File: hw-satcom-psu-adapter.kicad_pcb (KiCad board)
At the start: 2 copper layers, 89.2 x 45 mm, 37 parts, among them J1 Conn_01x04, J2 XT30, J3 XT30, J4 Conn_01x06_MountingPin, J5 s, U1 Brick-DCDC

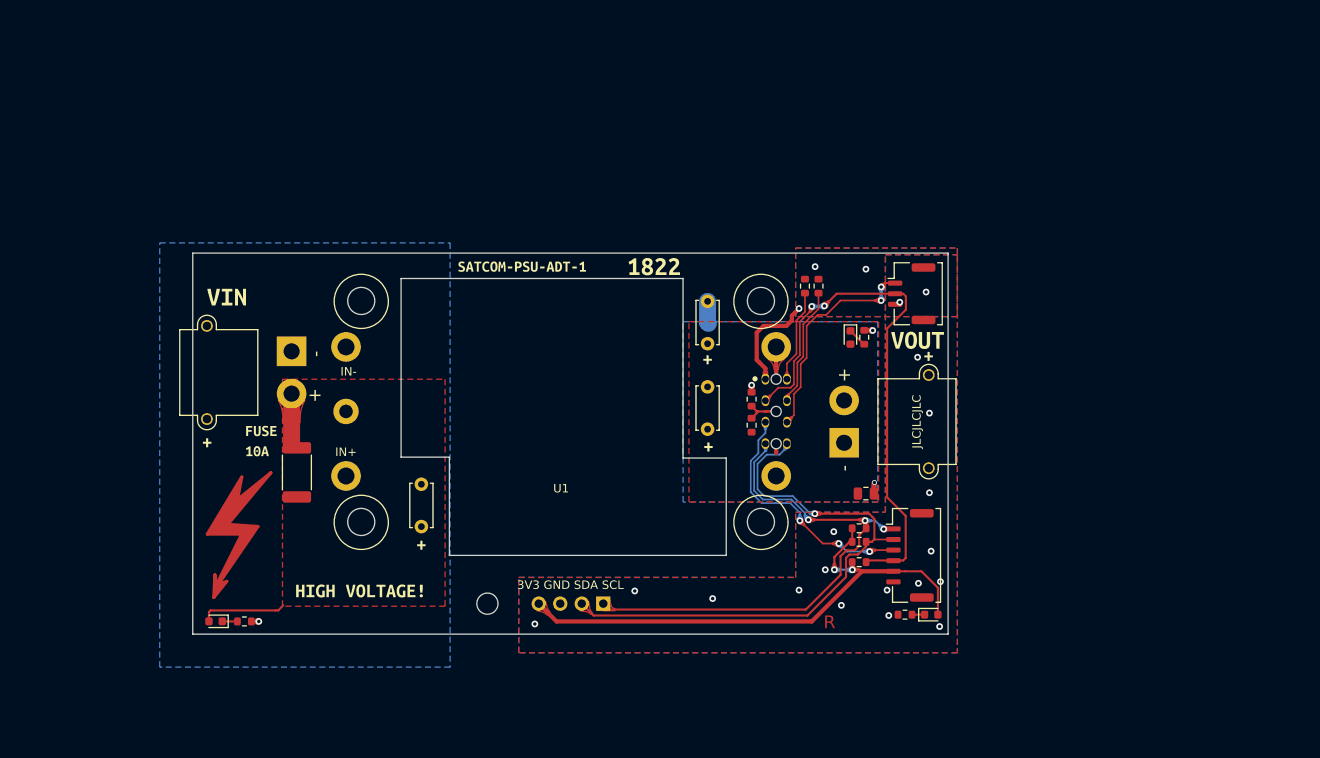
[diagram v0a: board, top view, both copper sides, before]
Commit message: ATX
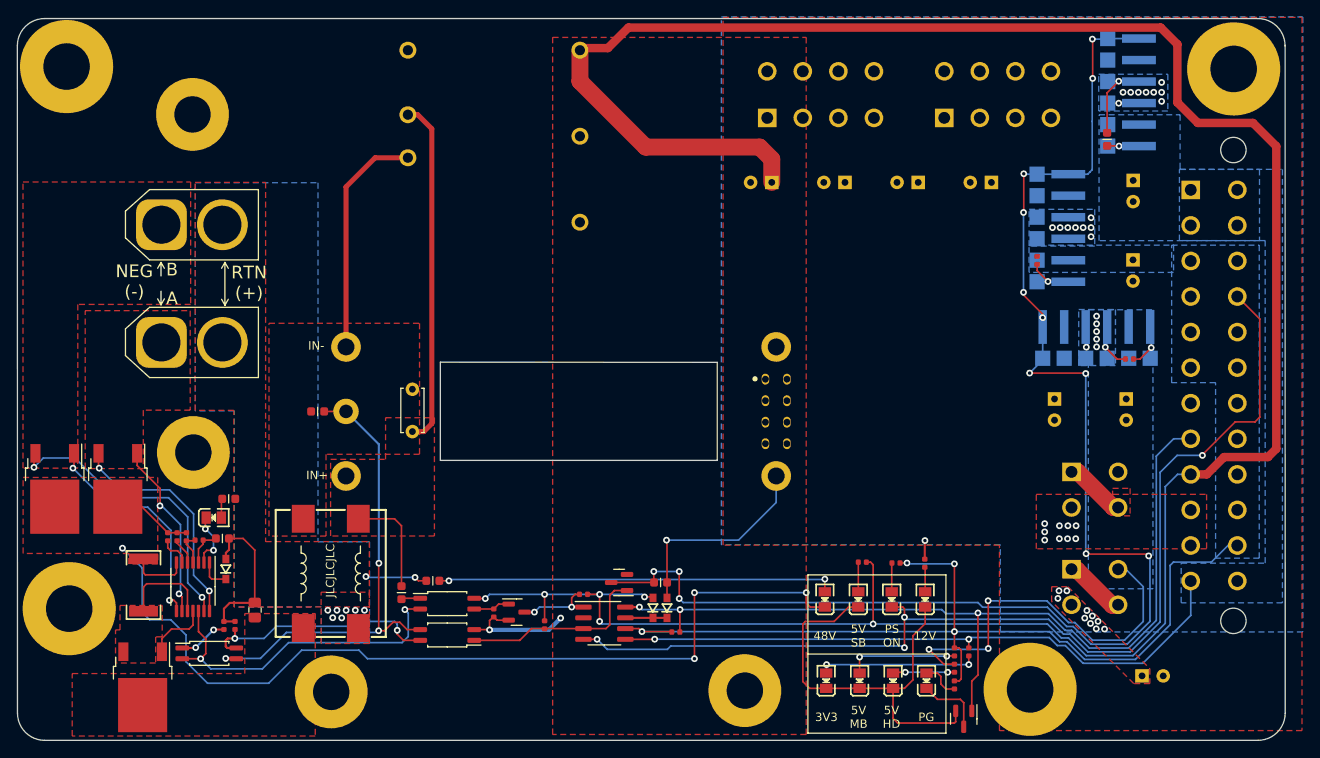
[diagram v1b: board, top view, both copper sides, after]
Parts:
- removed C2, C3: 470uF/50V, Capacitor_THT:C_Disc_D5.0mm_W2.5mm_P5.00mm
- removed C4: 1uF/50V, Capacitor_SMD:C_0805_2012Metric
- removed F1: 10A, Fuse:Fuse_2512_6332Metric
- removed H1: MountingHole, MountingHole:MountingHole_2.5mm
- removed R10, R9: NC, Resistor_SMD:R_0603_1608Metric
- removed REF**: Symbol_HighVoltage_Type1_CopperTop_Big, Symbol:Symbol_HighVoltage_Type1_CopperTop_Big
- removed kibuzzard-6276051F: G***, kibuzzard-6276051F
- removed kibuzzard-6276052C: G***, kibuzzard-6276052C
- removed kibuzzard-62760583 (x5): G***, kibuzzard-62760583
- removed kibuzzard-62760647: G***, kibuzzard-62760647
- removed kibuzzard-62760724: G***, kibuzzard-62760724
- removed kibuzzard-62760775: G***, kibuzzard-62760775
- added C10: 470uF/25V, Capacitor_THT:CP_Radial_D6.3mm_P2.50mm, B.Cu at (183.4, 69.8)
- added C12: 470uF/25V, Capacitor_THT:CP_Radial_D6.3mm_P2.50mm, B.Cu at (208.2, 95.4)
- added C13: 470uF/25V, Capacitor_THT:CP_Radial_D6.3mm_P2.50mm, B.Cu at (218.5, 128.1)
- added C14: 100nF/100V, lc:0805_C, F.Cu at (113.7, 120.4)
- added C15: 470uF/25V, Capacitor_THT:CP_Radial_D6.3mm_P2.50mm, B.Cu at (217.5, 69.6)
- added C16: 470uF/25V, Capacitor_THT:CP_Radial_D6.3mm_P2.50mm, B.Cu at (217.4, 79.0)
- added C17: 470uF/25V, Capacitor_THT:CP_Radial_D6.3mm_P2.50mm, B.Cu at (216.6, 95.4)
- added C5: 47nF, lc:0402_C, F.Cu at (104.5, 111.7)
- added C6: 10nF, lc:0402_C, F.Cu at (103.5, 111.7)
- added C7: 470uF/25V, Capacitor_THT:CP_Radial_D6.3mm_P2.50mm, B.Cu at (200.7, 69.8)
- added C8: 470uF/25V, Capacitor_THT:CP_Radial_D6.3mm_P2.50mm, B.Cu at (192.1, 69.8)
- added C9: 470uF/25V, Capacitor_THT:CP_Radial_D6.3mm_P2.50mm, B.Cu at (174.8, 69.8)
- added D10: Green, lc:0805_LED_S1_NUM, F.Cu at (189.1, 128.7)
- added D11: Blue, lc:0805_LED_S1_NUM, F.Cu at (193.1, 128.7)
- added D12: Blue, lc:0805_LED_S1_NUM, F.Cu at (188.9, 119.1)
- added D4: Yellow, lc:0805_LED_S1_NUM, F.Cu at (181.1, 119.1)
- added D5: Yellow, lc:0805_LED_S1_NUM, F.Cu at (185.0, 119.1)
- added D6: 1N5819WS, lc:SOD-323, F.Cu at (162.4, 120.1)
- added D7: 1N5819WS, lc:SOD-323, F.Cu at (160.8, 120.1)
- added D8: Green, lc:0805_LED_S1_NUM, F.Cu at (181.2, 128.7)
- added D9: Green, lc:0805_LED_S1_NUM, F.Cu at (185.2, 128.7)
- added FL1: ACM1513F-551T100, t123yh:ACM1513, F.Cu at (122.7, 116.0)
- added G***: LOGO, LOGO, F.Cu at (160.6, 93.1)
- added H2: SMTSO-M3, MountingHole:MountingHole_4.3mm_M4_Pad, B.Cu at (106.5, 101.8)
- added H3: SMTSO-M3, MountingHole:MountingHole_4.3mm_M4_Pad, B.Cu at (106.4, 61.8)
- added H4: SMTSO-632, MountingHole:MountingHole_5.5mm_Pad, B.Cu at (229.3, 56.5)
- added H5: SMTSO-632, MountingHole:MountingHole_5.5mm_Pad, B.Cu at (91.8, 120.2)
- added H6: SMTSO-632, MountingHole:MountingHole_5.5mm_Pad, B.Cu at (91.5, 56.2)
- added H7: SMTSO-632, MountingHole:MountingHole_5.5mm_Pad, B.Cu at (205.3, 129.7)
- added H8: SMTSO-M3, MountingHole:MountingHole_4.3mm_M4_Pad, F.Cu at (171.6, 129.9)
- added H9: SMTSO-M3, MountingHole:MountingHole_4.3mm_M4_Pad, F.Cu at (122.8, 130.0)
- added J_CPU1: Conn_02x04_Top_Bottom, t123yh:ATX-8P, B.Cu at (201.4, 59.5)
- added J_CPU2: Conn_02x04_Top_Bottom, t123yh:ATX-8P, B.Cu at (180.5, 59.5)
- added Q1: NCE0140K2, Package_TO_SOT_SMD:TO-252-2, F.Cu at (90.1, 106.0)
- added Q2: NCE0140K2, Package_TO_SOT_SMD:TO-252-2, F.Cu at (100.5, 129.5)
- added Q3: NCE0140K2, Package_TO_SOT_SMD:TO-252-2, F.Cu at (97.5, 106.0)
- added Q4: 2N7002, Package_TO_SOT_SMD:SOT-23, F.Cu at (144.7, 120.6)
- added Q5: 2N7002, Package_TO_SOT_SMD:SOT-23, F.Cu at (156.8, 117.1)
- added Q6: 2N7002, Package_TO_SOT_SMD:SOT-23, F.Cu at (197.4, 133.2)
- added R11: 8.2k, lc:0402_R, F.Cu at (105.7, 111.7)
- added R12: 220k, lc:0603_R, F.Cu at (110.7, 107.2)
- added R13: 51k, lc:0402_R, F.Cu at (110.1, 122.2)
- added R14: 120k, lc:0603_R, F.Cu at (134.8, 116.9)
- added R15: 3m, lc:2512_R, F.Cu at (100.6, 117.4)
- added R16: 10k, lc:0402_R, F.Cu at (111.4, 122.2)
- added R17: 220k, lc:0603_R, F.Cu at (121.2, 96.9)
- added R18: 51k, lc:0603_R, F.Cu at (131.1, 118.3)
- added R19: 22k, lc:0402_R, F.Cu at (141.9, 120.7)
- added R20: 5.1k, lc:0402_R, F.Cu at (147.9, 122.1)
- added R21: 5.1k, lc:0402_R, F.Cu at (152.6, 118.5)
- added R22: 8.2k, lc:0402_R, F.Cu at (185.5, 114.7)
- added R23: 22k, lc:0402_R, F.Cu at (163.4, 123.0)
- added R24: 10k, lc:0603_R, F.Cu at (161.7, 117.1)
- added R25: 390, lc:0603_R, F.Cu at (214.4, 64.8)
- added R26: 100, lc:0402_R, F.Cu at (206.1, 79.1)
- added R27: 100, lc:0402_R, F.Cu at (217.0, 90.7)
- added U10: ZXDN10, t123yh:ZXDN10, B.Cu at (206.8, 90.6)
- added U2: TPS2350, Package_SO:TSSOP-14_4.4x5mm_P0.65mm, F.Cu at (106.4, 117.6)
- added U3: EL3H7(B)(TA)-G, Package_SO:SOP-4_4.4x2.6mm_P1.27mm, F.Cu at (108.3, 125.5)
- added U4: EL3H7(B)(TA)-G, Package_SO:SOP-4_4.4x2.6mm_P1.27mm, F.Cu at (136.4, 123.3)
- added U5: AV10-48S05, t123yh:AV10-48Sxx, B.Cu at (141.9, 64.3)
- added U6: EL3H7(B)(TA)-G, Package_SO:SOP-4_4.4x2.6mm_P1.27mm, F.Cu at (136.4, 119.6)
- added U7: TPS3510, Package_SO:SOIC-8_3.9x4.9mm_P1.27mm, F.Cu at (155.0, 121.9)
- added U8: ZXDN10, t123yh:ZXDN10, B.Cu at (214.5, 52.9)
- added U9: ZXDN10, t123yh:ZXDN10, B.Cu at (206.1, 68.9)
- D1: value Yellow -> Green; footprint LED_SMD:LED_0603_1608Metric -> lc:0805_LED_S1_NUM
- D2: value Yellow -> Red; footprint LED_SMD:LED_0603_1608Metric -> lc:0805_LED_S1_NUM
- D3: value Yellow -> 1N4148WS; footprint LED_SMD:LED_0603_1608Metric -> lc:SOD-323
- J1: value Conn_01x04 -> Conn_01x02_Male; footprint Connector_PinSocket_2.54mm:PinSocket_1x04_P2.54mm_Vertical -> Connector_AMASS:AMASS_XT60-M_1x02_P7.20mm_Vertical; moved to F.Cu
- J2: value XT30 -> ATX-24; footprint Connector_AMASS:AMASS_XT30PW-M_1x02_P2.50mm_Horizontal -> t123yh:ATX-24P; moved to B.Cu
- J3: value XT30 -> Conn_02x02_Top_Bottom; footprint Connector_AMASS:AMASS_XT30PW-M_1x02_P2.50mm_Horizontal -> t123yh:ATX-4P; moved to B.Cu
- J4: value Conn_01x06_MountingPin -> Conn_02x02_Top_Bottom; footprint Connector_Molex:Molex_CLIK-Mate_502382-0670_1x06-1MP_P1.25mm_Vertical -> t123yh:ATX-4P; moved to B.Cu
- J5: value s -> Conn_01x02_Male; footprint Connector_Molex:Molex_CLIK-Mate_502382-0370_1x03-1MP_P1.25mm_Vertical -> Connector_AMASS:AMASS_XT60-M_1x02_P7.20mm_Vertical
- R1: value 4.7k -> 200k; footprint Resistor_SMD:R_0603_1608Metric -> lc:0402_R
- R2: value 4.7k -> 22k; footprint Resistor_SMD:R_0603_1608Metric -> lc:0402_R
- R3: value 4.7k -> 56k; footprint Resistor_SMD:R_0603_1608Metric -> lc:0402_R
- R4: value 3.9k -> 56k; footprint Resistor_SMD:R_0603_1608Metric -> lc:0402_R
- R5: value 100k -> 390k; footprint Resistor_SMD:R_0603_1608Metric -> lc:0603_R
- R6: value 47k -> 5.6k; footprint Resistor_SMD:R_0603_1608Metric -> lc:0402_R
- R7, R8: value NC -> 3.3k; footprint Resistor_SMD:R_0603_1608Metric -> lc:0402_R
- kibuzzard-62760563: moved to B.Cu
- moved J2 109.0 mm to (227.0, 93.8)
- moved J5 89.0 mm to (102.7, 74.8), turned to 0 degrees
- moved R6 82.1 mm to (107.2, 112.1), turned to 180 degrees
- moved D3 78.7 mm to (110.3, 115.5), turned to 90 degrees
- moved J1 60.6 mm to (102.7, 88.8), turned to 0 degrees
- moved R7 50.3 mm to (196.3, 129.2)
- moved R8 34.0 mm to (189.4, 114.8), turned to 0 degrees
- moved kibuzzard-62760563 32.8 mm to (97.1, 133.4)
- moved J3 30.1 mm to (212.9, 106.1), turned to 90 degrees
- moved J4 22.1 mm to (212.9, 117.6), turned to 90 degrees
- moved R2 19.5 mm to (198.1, 125.3), turned to 90 degrees
- moved R3 15.5 mm to (196.3, 125.3), turned to 90 degrees
- moved D2 12.2 mm to (108.9, 109.4), turned to 0 degrees
- moved C1 11.3 mm to (132.3, 99.3)
- moved R5 10.1 mm to (109.9, 111.9), turned to 180 degrees
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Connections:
- C1 pad 1: /VIN -> /RTN_FIL
- C1 pad 2: GND1 -> /NEG_FIL
- D1 pad 1: Net-(D1-Pad1) -> GND2
- D1 pad 2: +3V3 -> Net-(D1-Pad2)
- D2 pad 2: /VIN -> Net-(D2-Pad2)
- D3 pad 2: /VOUT -> /RTN
- J1 pad 1: I2C_SCL -> /NEGA
- J1 pad 2: I2C_SDA -> /RTN
- J2 pad 1: GND1 -> +3.3V
- J2 pad 2: Net-(F1-Pad1) -> +3.3V
- J3 pad 2: /VOUT -> +12V
- J4 pad 1: I2C_SCL -> GND2
- J4 pad 2: I2C_SDA -> +12V
- J4 pad 3: PMBus_CTL -> +5VD
- J4 pad 4: PMBus_ALT -> GND2
- J5 pad 1: Net-(J5-Pad1) -> /NEGB
- J5 pad 2: PMBus_ALT -> /RTN
- R1 pad 1: +3V3 -> Net-(D1-Pad2)
- R1 pad 2: I2C_SDA -> +12V
- R2 pad 1: +3V3 -> Net-(D8-Pad2)
- R2 pad 2: I2C_SCL -> +3.3V
- R3 pad 1: +3V3 -> Net-(D9-Pad2)
- R3 pad 2: PMBus_ALT -> +5VA
- R4 pad 1: Net-(D1-Pad1) -> Net-(D10-Pad2)
- R4 pad 2: GNDS -> +5VD
- R5 pad 1: Net-(D2-Pad1) -> /RTN
- R5 pad 2: GND1 -> Net-(R5-Pad2)
- R6 pad 1: Net-(D3-Pad1) -> Net-(R5-Pad2)
- R6 pad 2: GND2 -> Net-(R11-Pad1)
- R7 pad 1: Net-(R7-Pad1) -> Net-(D11-Pad2)
- R7 pad 2: GNDS -> +5VA
- R8 pad 1: GNDS -> Net-(D12-Pad2)
- R8 pad 2: Net-(R8-Pad2) -> +5VA
- U1 pad 2: Net-(R7-Pad1) -> unconnected-(U1-Pad2)
- U1 pad 4: Net-(R8-Pad2) -> unconnected-(U1-Pad4)
- U1 pad 6: Net-(J5-Pad1) -> unconnected-(U1-Pad6)
- U1 pad GATE: /VIN -> Net-(R17-Pad2)
- U1 pad IN+: /VIN -> /RTN_FIL
- U1 pad IN-: GND1 -> /NEG_FIL
- U1 pad OUT+: /VOUT -> +12V
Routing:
- net /+5VSB: track 0.00 -> 300.1 mm, vias 0 -> 6
- net /DCDC_EN: track 0.00 -> 168.1 mm, vias 0 -> 13
- net /PSON: track 0.00 -> 125.7 mm, vias 0 -> 4
- net /NEG: track 0.00 -> 122.1 mm, vias 0 -> 4
- net +5VA: track 0.00 -> 108.6 mm, vias 0 -> 4
- net /PGOOD: track 0.00 -> 104.9 mm, vias 0 -> 3
- net GND2: track 8.51 -> 88.3 mm, vias 3 -> 27
- net +3.3V: track 0.00 -> 75.5 mm, vias 0 -> 2
- net I2C_SDA: track 68.1 -> 0.00 mm, vias 1 -> 0
- net +3V3: track 64.6 -> 0.00 mm, vias 2 -> 0
- net PMBus_ALT: track 63.7 -> 0.00 mm, vias 2 -> 0
- net I2C_SCL: track 63.0 -> 0.00 mm, vias 3 -> 0
- net Net-(R17-Pad2): track 0.00 -> 56.5 mm, vias 0 -> 3
- net /RTN_FIL: track 0.00 -> 53.6 mm
- net Net-(D4-Pad2): track 0.00 -> 47.1 mm, vias 0 -> 2
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- added copper zone on B.Cu, net +12V
- added copper zone on F.Cu, net +12V
- added copper zone on B.Cu, net +3.3V
- added copper zone on B.Cu, net +5VA
- added copper zone on B.Cu, net +5VD
- added copper zone on F.Cu, net /NEG
- added copper zone on F.Cu, net /NEGA
- added copper zone on F.Cu, net /NEGB
- added copper zone on F.Cu, net /NEG_FIL
- added copper zone on F.Cu, net /NEG_SS
- added copper zone on B.Cu, net /RTN
- added copper zone on F.Cu, net /RTN
- added copper zone on F.Cu, net /RTN_FIL
- added copper zone on F.Cu, net GND2
- added copper zone on F.Cu, net Net-(Q2-Pad3)
- removed copper zone on F.Cu, net /VIN
- removed copper zone on F.Cu, net /VOUT
- removed copper zone on B.Cu, net GND1
- removed copper zone on B.Cu, net GNDS
- removed copper zone on F.Cu, net GNDS
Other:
- board size 89.2 x 45 mm -> 149.7 x 85.2 mm
- board text added: "12V"
- board text added: "3V3"
- board text added: "48V"
- board text added: "5V"
- board text added: "5V HD"
- board text added: "5V MB"
- board text added: "5V SB"
- board text added: "5VSB"
- board text added: "A"
- board text added: "B"
- board text added: "GND"
- board text added: "HDD Power"
- board text added: "NC"
- board text added: "NEG (-)"
- board text added: "PG"
- board text added: "PS ON"
- board text added: "PSON"
- board text added: "RTN (+)"
- board text removed: "3V3 GND SDA SCL"
- board text removed: "R"
